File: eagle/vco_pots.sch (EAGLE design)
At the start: 17 parts, among them P1 P0915N, P10 P0915N, P2 P0915N, P3 P0915N, P4 P0915N, P5 P0915N, P6 P0915N, P7 P0915N, P8 P0915N, P9 P0915N, X1 87758-1416, X2 87758-0216, X3 87758-0216

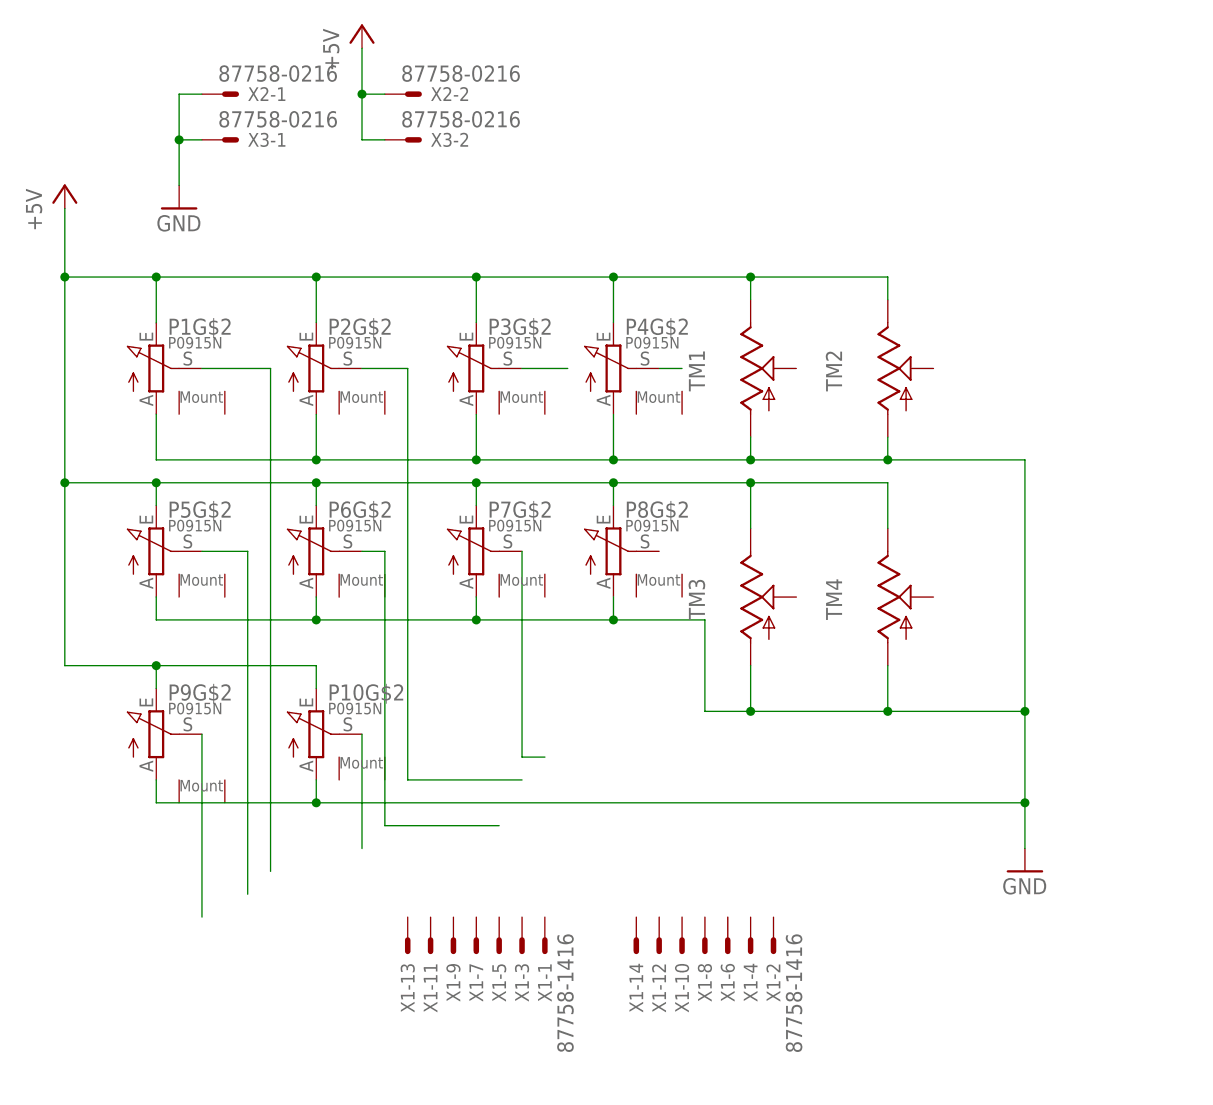
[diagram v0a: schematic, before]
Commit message: schemo wired
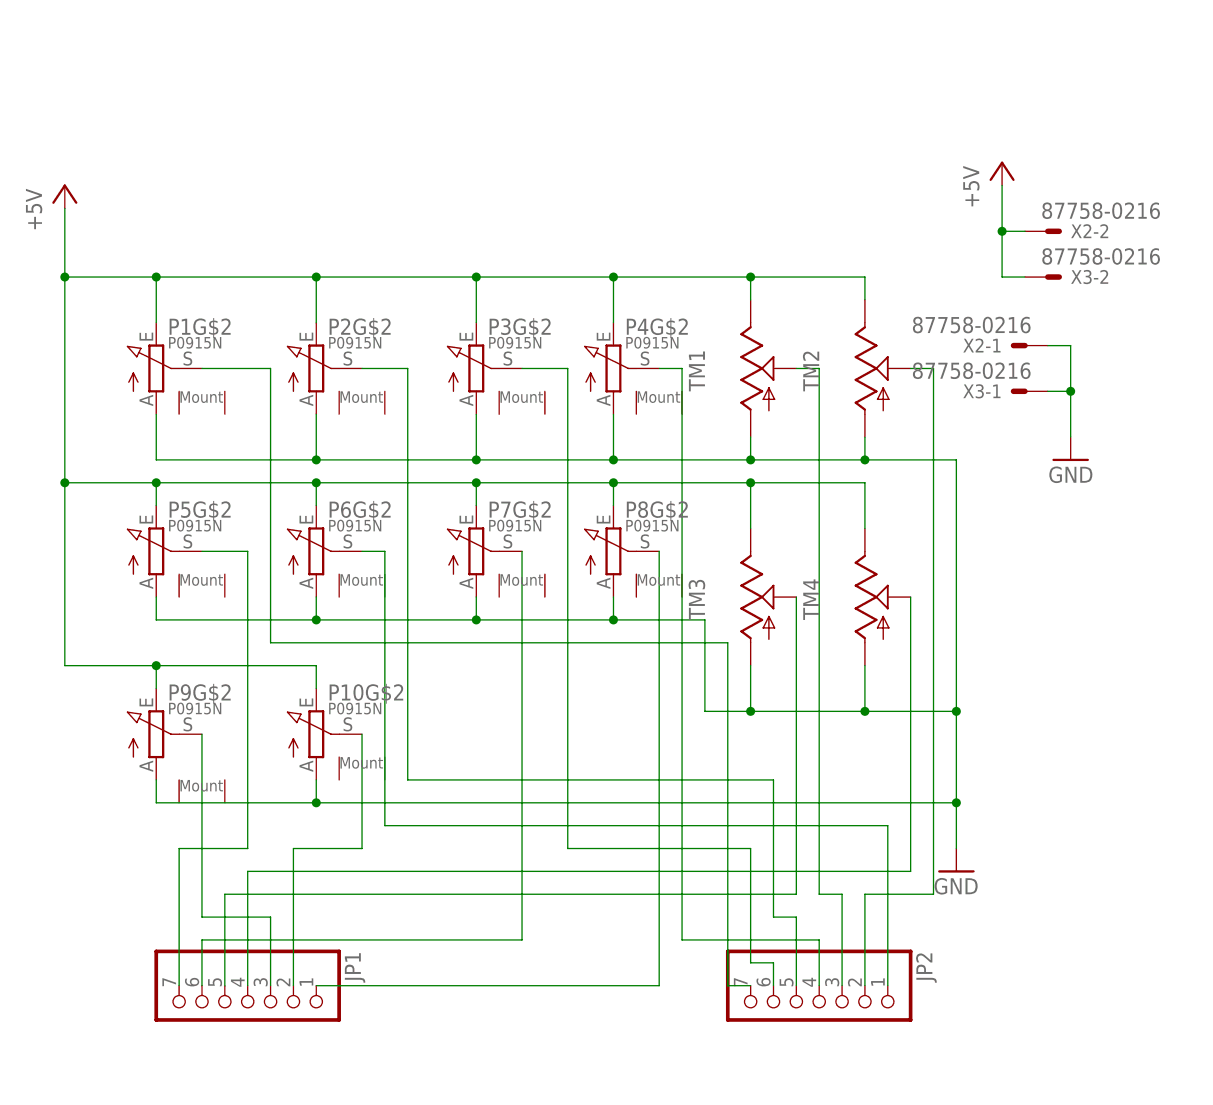
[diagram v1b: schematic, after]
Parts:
- removed X1: 87758-1416, con-molex:87758-1416
- added JP1, JP2: (no value), pinhead:PINHD-1X7
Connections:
- new net N$11: JP1.4, TM4.WIPER
- new net N$12: JP1.5, TM3.WIPER
- new net N$13: JP2.2, TM2.WIPER
- new net N$14: JP2.3, TM1.WIPER
- new net N$6: JP1.1, P8G$2.S
- net N$1: now also JP1.2
- net N$10: now also JP2.4
- net N$2: now also JP2.1
- net N$3: now also JP2.5
- net N$4: now also JP1.6
- net N$5: now also JP2.6
- net N$7: now also JP1.3
- net N$8: now also JP1.7
- net N$9: now also JP2.7
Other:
- moved on the sheet: TM2, TM4, X2-1, X2-2, X3-1, X3-2
